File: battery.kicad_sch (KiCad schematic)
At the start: 86 parts, among them J6 Conn_01x02, Q3 AON7534, Q4 AON7534, Q7 TI CSD18512Q5B, SW3 RESET, U10 MAX17320G22+, U9 BQ25798

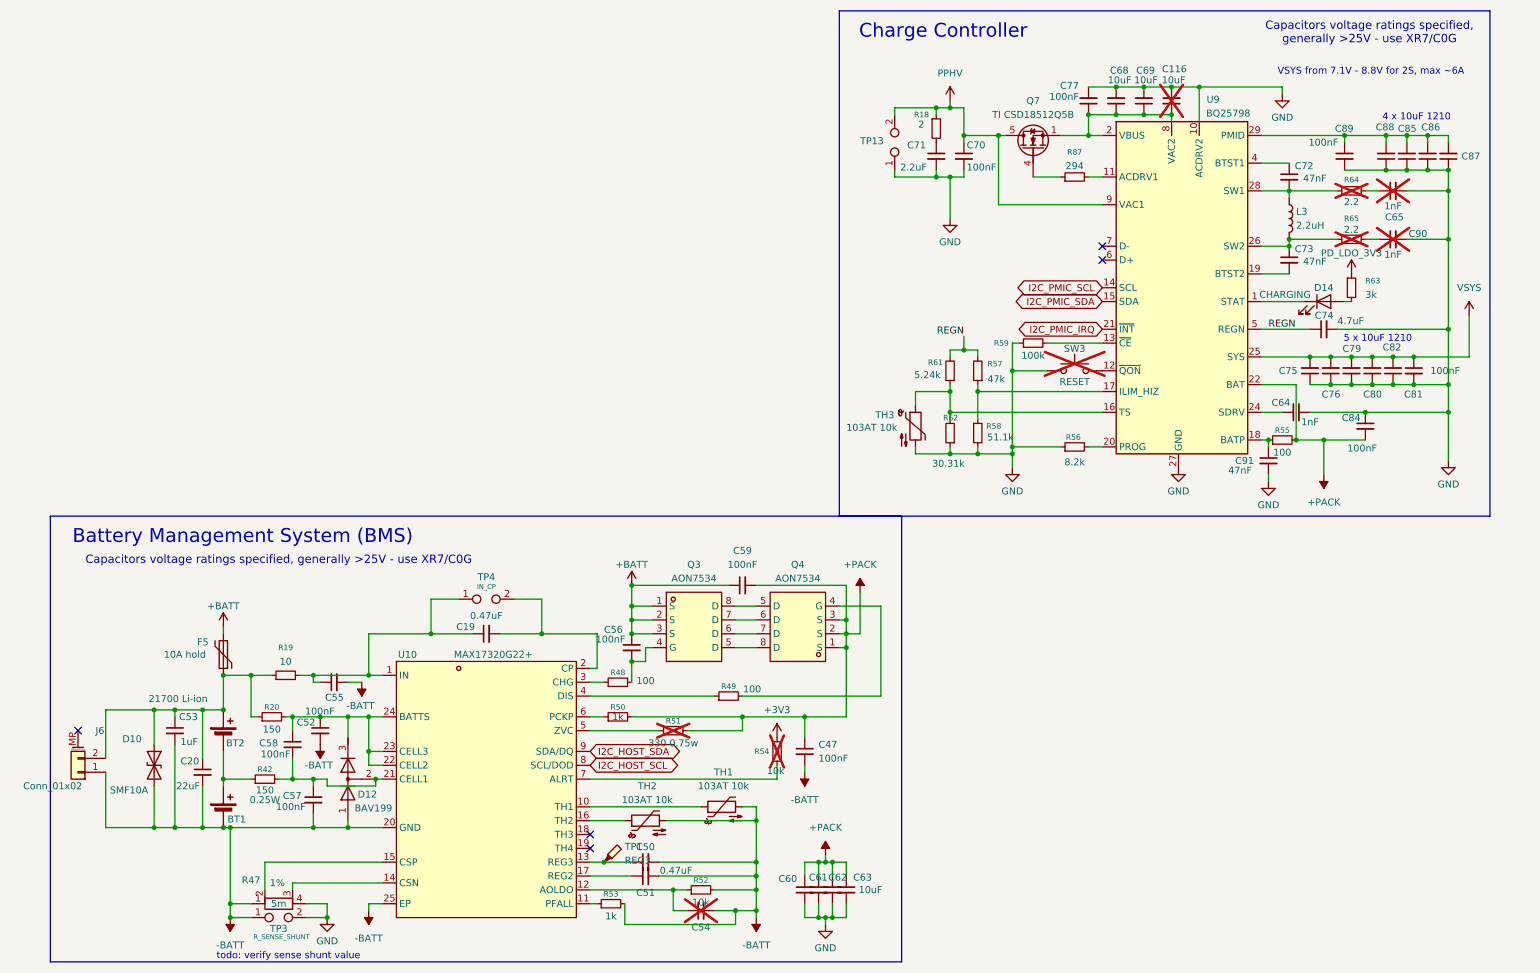
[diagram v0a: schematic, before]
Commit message: push for review, minor changes
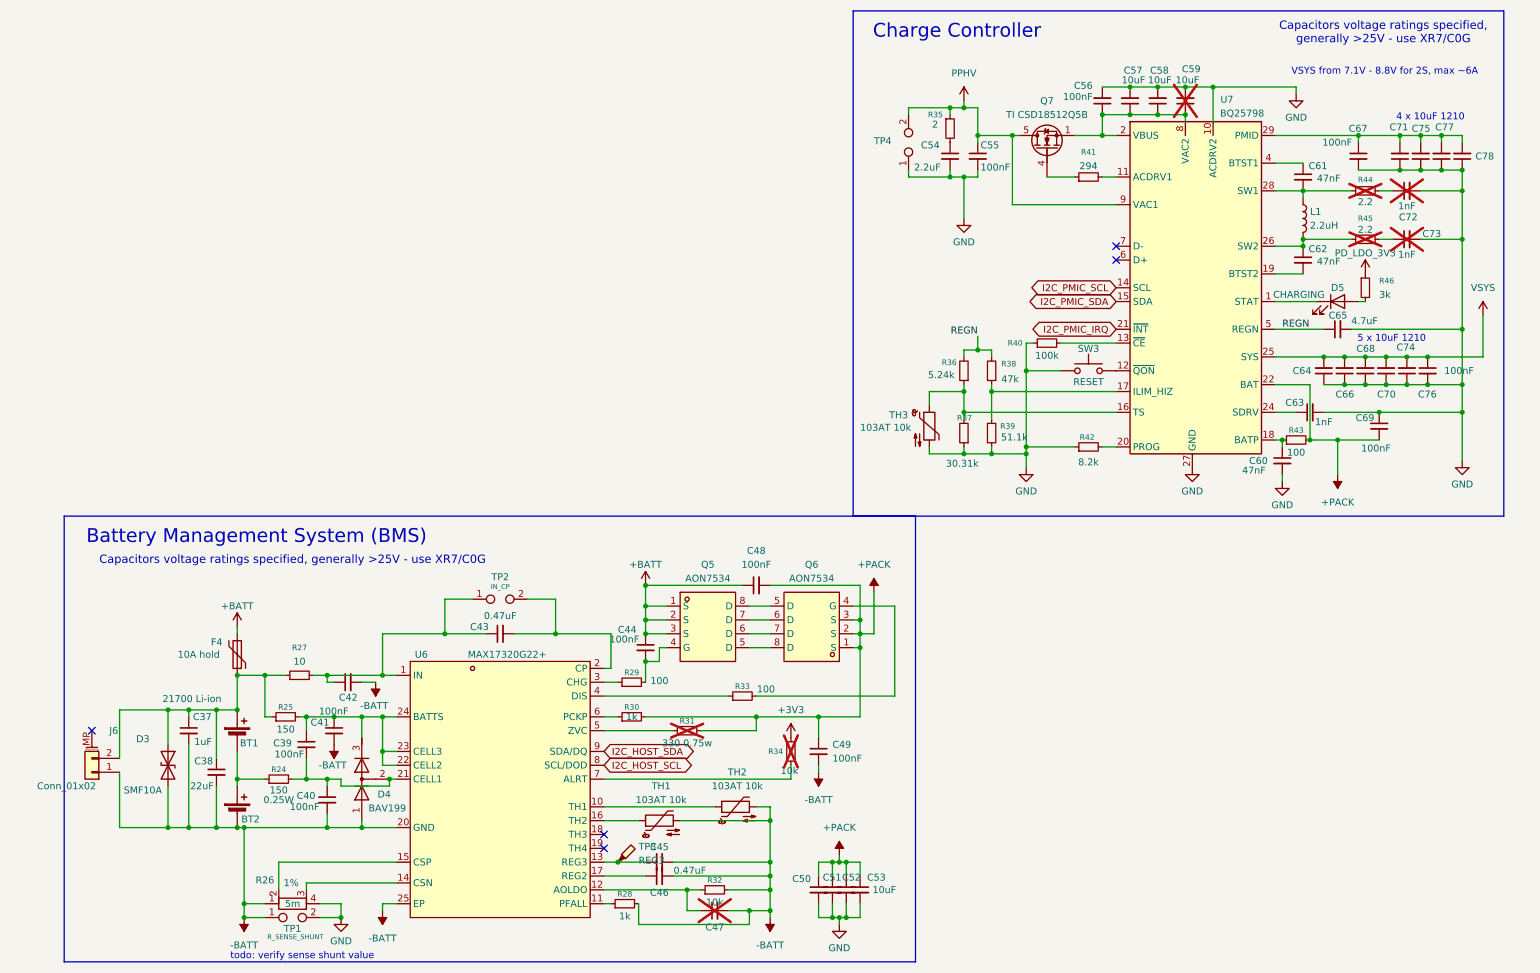
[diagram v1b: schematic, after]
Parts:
- removed C116, C79, C80, C82, C85, C86, C87, C88: 10uF, Capacitor_SMD:C_1210_3225Metric, symbol Device:C_Small
- removed C19: 0.47uF, symbol Device:C_Small
- removed C20: 22uF, Capacitor_SMD:C_0805_2012Metric, symbol Device:C_Small
- removed C81, C84, C89: 100nF, Capacitor_SMD:C_0402_1005Metric, symbol Device:C_Small
- removed C90: 1nF, Capacitor_SMD:C_0402_1005Metric_Pad0.74x0.62mm_HandSolder, symbol Device:C_Small
- removed C91: 47nF, Capacitor_SMD:C_0402_1005Metric, symbol Device:C_Small
- removed D10: SMF10A, Diode_SMD:D_SOD-123, symbol Device:D_TVS
- removed D12: BAV199, Package_TO_SOT_SMD:SOT-23, symbol Device:D_Dual_Series_ACK
- removed D14: CHARGING, symbol Device:LED
- removed F5: 10A hold, symbol Device:Polyfuse
- removed L3: 2.2uH, symbol Device:L
- removed Q3, Q4: AON7534, easyeda2kicad:PQFN-8_L3.1-W3.1-P0.65-LS3.3-BL, symbol easyeda2kicad:AON7534-ES
- removed R18: 2, Resistor_SMD:R_0402_1005Metric, symbol Device:R_Small
- removed R19: 10, symbol Device:R_Small
- removed R20: 150, Resistor_SMD:R_1206_3216Metric, symbol Device:R_Small
- removed R47: 5m, symbol Device:R_Shunt
- removed R48, R49: 100, symbol Device:R_Small
- removed R50, R53: 1k, symbol Device:R_Small
- removed R51: 330 0.75w, Resistor_SMD:R_2010_5025Metric, symbol Device:R_Small
- removed R52, R54: 10k, symbol Device:R_Small
- removed R55: 100, Resistor_SMD:R_0402_1005Metric, symbol Device:R_Small
- removed R56: 8.2k, Resistor_SMD:R_0402_1005Metric_Pad0.72x0.64mm_HandSolder, symbol Device:R_Small
- removed R57: 47k, Resistor_SMD:R_0603_1608Metric_Pad0.98x0.95mm_HandSolder, symbol Device:R_Small
- removed R58: 51.1k, Resistor_SMD:R_0603_1608Metric_Pad0.98x0.95mm_HandSolder, symbol Device:R_Small
- removed R59: 100k, Resistor_SMD:R_0402_1005Metric, symbol Device:R_Small
- removed R61: 5.24k, Resistor_SMD:R_0603_1608Metric_Pad0.98x0.95mm_HandSolder, symbol Device:R_Small
- removed R62: 30.31k, Resistor_SMD:R_0603_1608Metric_Pad0.98x0.95mm_HandSolder, symbol Device:R_Small
- removed R63: 3k, Resistor_SMD:R_0402_1005Metric_Pad0.72x0.64mm_HandSolder, symbol Device:R_Small
- removed R64, R65: 2.2, Resistor_SMD:R_0402_1005Metric_Pad0.72x0.64mm_HandSolder, symbol Device:R_Small
- removed R87: 294, symbol Device:R_Small
- removed TP1: REG3, symbol Connector:TestPoint_Probe
- removed TP13: PPHV, symbol Connector:TestPoint_2Pole
- removed TP3: R_SENSE_SHUNT, TestPoint:TestPoint_2Pads_Pitch2.54mm_Drill0.8mm, symbol Connector:TestPoint_2Pole
- removed U10: MAX17320G22+, easyeda2kicad:QFN-24_L4.0-W4.0-P0.50-BL-EP2.6, symbol easyeda2kicad:MAX17320G22+
- removed U9: BQ25798, Package_DFN_QFN:Texas_RQM0029A_VQFN-29_4x4mm_P0.4mm, symbol Battery_Management:BQ25798
- added C37, C42: 1uF, symbol Device:C_Small
- added C38: 22uF, Capacitor_SMD:C_0805_2012Metric, symbol Device:C_Small
- added C39, C40, C41, C44, C48, C49: 100nF, symbol Device:C_Small
- added C43: 0.47uF, symbol Device:C_Small
- added C45, C46: 0.47uF, Capacitor_SMD:C_0402_1005Metric, symbol Device:C_Small
- added C66, C78: 10uF, Capacitor_SMD:C_1210_3225Metric, symbol Device:C_Small
- added C67: 100nF, Capacitor_SMD:C_0402_1005Metric, symbol Device:C_Small
- added D3: SMF10A, Diode_SMD:D_SOD-123, symbol Device:D_TVS
- added D4: BAV199, Package_TO_SOT_SMD:SOT-23, symbol Device:D_Dual_Series_ACK
- added D5: CHARGING, symbol Device:LED
- added F4: 10A hold, symbol Device:Polyfuse
- added L1: 2.2uH, Inductor_SMD:L_Vishay_IFSC-1515AH_4x4x1.8mm, symbol Device:L
- added Q5, Q6: AON7534, easyeda2kicad:PQFN-8_L3.1-W3.1-P0.65-LS3.3-BL, symbol easyeda2kicad:AON7534-ES
- added R24, R25: 150, Resistor_SMD:R_1206_3216Metric, symbol Device:R_Small
- added R26: 5m, symbol Device:R_Shunt
- added R27: 10, symbol Device:R_Small
- added R28, R30: 1k, symbol Device:R_Small
- added R29, R33: 100, symbol Device:R_Small
- added R31: 330 0.75w, Resistor_SMD:R_2010_5025Metric, symbol Device:R_Small
- added R32, R34: 10k, symbol Device:R_Small
- added R35: 2, Resistor_SMD:R_0402_1005Metric, symbol Device:R_Small
- added R36: 5.24k, Resistor_SMD:R_0603_1608Metric_Pad0.98x0.95mm_HandSolder, symbol Device:R_Small
- added R37: 30.31k, Resistor_SMD:R_0603_1608Metric_Pad0.98x0.95mm_HandSolder, symbol Device:R_Small
- added R38: 47k, Resistor_SMD:R_0603_1608Metric_Pad0.98x0.95mm_HandSolder, symbol Device:R_Small
- added R39: 51.1k, Resistor_SMD:R_0603_1608Metric_Pad0.98x0.95mm_HandSolder, symbol Device:R_Small
- added R40: 100k, Resistor_SMD:R_0402_1005Metric, symbol Device:R_Small
- added R41: 294, symbol Device:R_Small
- added R43: 100, Resistor_SMD:R_0402_1005Metric, symbol Device:R_Small
- added R44, R45: 2.2, Resistor_SMD:R_0402_1005Metric_Pad0.72x0.64mm_HandSolder, symbol Device:R_Small
- added R46: 3k, Resistor_SMD:R_0402_1005Metric_Pad0.72x0.64mm_HandSolder, symbol Device:R_Small
- added TP1: R_SENSE_SHUNT, TestPoint:TestPoint_2Pads_Pitch2.54mm_Drill0.8mm, symbol Connector:TestPoint_2Pole
- added TP2: IN_CP, TestPoint:TestPoint_2Pads_Pitch2.54mm_Drill0.8mm, symbol Connector:TestPoint_2Pole
- added TP3: REG3, symbol Connector:TestPoint_Probe
- added U6: MAX17320G22+, easyeda2kicad:QFN-24_L4.0-W4.0-P0.50-BL-EP2.6, symbol easyeda2kicad:MAX17320G22+
- added U7: BQ25798, Package_DFN_QFN:Texas_RQM0029A_VQFN-29_4x4mm_P0.4mm, symbol Battery_Management:BQ25798
- C47: value 100nF -> 0.47uF; footprint (none) -> Capacitor_SMD:C_0402_1005Metric; Voltage Rating 50V -> 16V; now not fitted
- C50: value 0.47uF -> 10uF; footprint Capacitor_SMD:C_0402_1005Metric -> Capacitor_SMD:C_0805_2012Metric; LCSC Part (none) -> C33546010
- C51: value 0.47uF -> 10uF; footprint Capacitor_SMD:C_0402_1005Metric -> Capacitor_SMD:C_0805_2012Metric; LCSC Part (none) -> C33546010; Voltage Rating 16V -> 25V
- C52: value 100nF -> 10uF; footprint (none) -> Capacitor_SMD:C_0805_2012Metric; LCSC Part (none) -> C33546010; Voltage Rating 50V -> 25V
- C53: value 1uF -> 10uF; footprint (none) -> Capacitor_SMD:C_0805_2012Metric; LCSC Part (none) -> C33546010; Voltage Rating 50V -> 25V
- C54: value 0.47uF -> 2.2uF; footprint Capacitor_SMD:C_0402_1005Metric -> Capacitor_SMD:C_0805_2012Metric; Voltage Rating 16V -> 50V; now fitted
- C55: value 1uF -> 100nF; footprint (none) -> Capacitor_SMD:C_0402_1005Metric; LCSC Part (none) -> C6119785
- C56: footprint (none) -> Capacitor_SMD:C_0402_1005Metric; LCSC Part (none) -> C6119785; Voltage Rating 25V -> 50V
- C57: value 100nF -> 10uF; footprint (none) -> Capacitor_SMD:C_1210_3225Metric; LCSC Part (none) -> C33546018; Voltage Rating 25V -> 50V
- C58: value 100nF -> 10uF; footprint (none) -> Capacitor_SMD:C_1210_3225Metric; LCSC Part (none) -> C33546018
- C59: value 100nF -> 10uF; footprint (none) -> Capacitor_SMD:C_1210_3225Metric; LCSC Part (none) -> C33546018; now not fitted
- C60, C61, C62: value 10uF -> 47nF; footprint Capacitor_SMD:C_0805_2012Metric -> Capacitor_SMD:C_0402_1005Metric; LCSC Part C33546010 -> (none); Voltage Rating 25V -> 50V
- C63: value 10uF -> 1nF; footprint Capacitor_SMD:C_0805_2012Metric -> Capacitor_SMD:C_0402_1005Metric; LCSC Part C33546010 -> (none); Voltage Rating 25V -> 50V
- C64: value 1nF -> 10uF; footprint Capacitor_SMD:C_0402_1005Metric -> Capacitor_SMD:C_1210_3225Metric; LCSC Part (none) -> C7472976
- C65: value 1nF -> 4.7uF; footprint Capacitor_SMD:C_0402_1005Metric_Pad0.74x0.62mm_HandSolder -> Capacitor_SMD:C_0603_1608Metric; Voltage Rating 50V -> 16V; now fitted; now in the parts list
- C68: LCSC Part C33546018 -> C7472976
- C69: value 10uF -> 100nF; footprint Capacitor_SMD:C_1210_3225Metric -> Capacitor_SMD:C_0402_1005Metric; LCSC Part C33546018 -> C6119785
- C70, C77: value 100nF -> 10uF; footprint Capacitor_SMD:C_0402_1005Metric -> Capacitor_SMD:C_1210_3225Metric; LCSC Part C6119785 -> C7472976
- C71: value 2.2uF -> 10uF; footprint Capacitor_SMD:C_0805_2012Metric -> Capacitor_SMD:C_1210_3225Metric; LCSC Part (none) -> C7472976
- C72, C73: value 47nF -> 1nF; footprint Capacitor_SMD:C_0402_1005Metric -> Capacitor_SMD:C_0402_1005Metric_Pad0.74x0.62mm_HandSolder; now not fitted; now left out of the parts list
- C74: value 4.7uF -> 10uF; footprint Capacitor_SMD:C_0603_1608Metric -> Capacitor_SMD:C_1210_3225Metric; LCSC Part (none) -> C7472976; Voltage Rating 16V -> 50V
- C76: value 10uF -> 100nF; footprint Capacitor_SMD:C_1210_3225Metric -> Capacitor_SMD:C_0402_1005Metric; LCSC Part C7472976 -> C6119785
- R42: value 150 -> 8.2k; footprint Resistor_SMD:R_1206_3216Metric -> Resistor_SMD:R_0402_1005Metric_Pad0.72x0.64mm_HandSolder; Power Rating 0.25W -> (none); Tolerance (none) -> 1%
- SW3: now fitted
- TP4: value IN_CP -> PPHV; footprint TestPoint:TestPoint_2Pads_Pitch2.54mm_Drill0.8mm -> (none)
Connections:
- net +3V3: now also R34.2
- net +BATT: now also C44.1, C48.1, F4.2, Q5.1 (S), Q5.2 (S), Q5.3 (S); no longer C56.1, C59.1
- net +PACK: now also C50.1, C51.1, C52.1, C53.1, C69.2, C48.2, C49.1, Q6.1 (S), Q6.2 (S), Q6.3 (S), R30.2, R31.2, R43.2, U7.22 (BAT), U7.23 (BAT); no longer C47.1, C59.2, C60.1, C61.1, C62.1, C63.1
- net -BATT: now also BT2.2 (-), C37.2, C38.2, C40.2, C41.2, C42.2, C45.2, C46.2, C49.2, D3.2 (A2), D4.1 (A), R26.1, R28.2, R32.2, TP1.1, U6.20 (GND), U6.25 (EP); no longer BT1.2 (-), C50.2, C51.2, C52.2, C53.2, C54.2, C55.2, C57.2
- net GND: now also C50.2, C51.2, C52.2, C53.2, C54.2, C55.2, C56.2, C57.2, C58.2, C59.2, C64.1, C68.1, C69.1, C70.1, C71.1, C72.2, C73.2, C74.1, C76.2, C77.1, R42.1, TP4.1, C66.1, C67.2, C78.1, R26.4, R37.1, R39.2, R40.1, TP1.2, U7.10 (ACDRV2), U7.27 (GND); no longer C61.2, C62.2, C64.2, C68.2, C69.2, C70.2, C71.2, C74.2, C76.1, C77.2
- net I2C_HOST_SCL: now also U6.8 (SCL/DOD)
- net I2C_HOST_SDA: now also U6.9 (SDA/DQ)
- net I2C_PMIC_IRQ: now also U7.21 (~{INT})
- net I2C_PMIC_SCL: now also U7.14 (SCL)
- net I2C_PMIC_SDA: now also U7.15 (SDA)
- net PD_LDO_3V3: now also R46.1
- net PPHV: now also C55.1, TP4.2, R35.1, U7.9 (VAC1); no longer C70.1
- net REGN: now also C65.1, R36.2, R38.2, U7.5 (REGN); no longer C74.1
- net VSYS: now also C64.2, C68.2, C70.2, C74.2, C76.1, C66.2, U7.25 (SYS); no longer C75.2, C76.2
- net at Q7.1 (S), Q7.2 (S), Q7.3 (S): now also C56.1, C57.1, C58.1, C59.1, U7.2 (VBUS), U7.3 (VBUS), U7.8 (VAC2); no longer C68.1, C69.1, C77.1
- net at Q7.4 (G): now also R41.1
- net at TH3.1: now also R36.1, R37.2, U7.16 (TS)
- net at TH1.1: now also U6.16 (TH2)
- net at SW3.2: now also U7.12 (~{QON})
- net at C72.1: now also R44.2
- net at C54.1: now also R35.2
- net at C73.1: now also R45.2
- net at TH2.1: now also U6.10 (TH1)
- new net: R26.2, U6.15 (CSP)
- new net: R26.3, U6.14 (CSN)
- new net: C60.1, R43.1, U7.18 (BATP)
- new net: C45.1, TP3.1, U6.13 (REG3)
- new net: BT1.1 (+), C37.1, C38.1, D3.1 (A1), F4.1, J6.2 (Pin_2), R25.1, R27.1
- new net: C62.1, L1.2, R45.1, U7.26 (SW2)
- new net: R40.2, U7.13 (~{CE})
- new net: C39.2, C40.1, D4.2 (common), R24.2, U6.21 (CELL1)
- new net: C39.1, C41.1, D4.3 (K), R25.2, U6.22 (CELL2), U6.23 (CELL3), U6.24 (BATTS)
- new net: R31.1, U6.5 (ZVC)
- new net: BT1.2 (-), BT2.1 (+), R24.1
- new net: C63.1, U7.24 (SDRV)
- new net: C62.2, U7.19 (BTST2)
- new net: C42.1, C43.1, R27.2, TP2.1, U6.1 (IN)
- new net: R28.1, U6.11 (PFALL)
- new net: C47.1, R32.1, U6.12 (AOLDO)
- new net: C46.1, U6.17 (REG2)
- new net: C43.2, TP2.2, U6.2 (CP)
- new net: R29.1, U6.3 (CHG)
- new net: R33.1, U6.4 (DIS)
- new net: R30.1, U6.6 (PCKP)
- new net: R34.1, U6.7 (ALRT)
- new net: C67.1, C71.2, C75.2, C77.2, C78.2, U7.29 (PMID)
- new net: Q6.4 (G), R33.2
- new net: Q5.8 (D), Q6.5 (D)
- new net: Q5.7 (D), Q6.6 (D)
- new net: Q5.6 (D), Q6.7 (D)
- new net: Q5.5 (D), Q6.8 (D)
- new net: R38.1, R39.1, U7.17 (ILIM_HIZ)
- new net: D5.1 (K), U7.1 (STAT)
- new net: R41.2, U7.11 (ACDRV1)
- new net: R42.2, U7.20 (PROG)
- new net: C61.2, L1.1, R44.1, U7.28 (SW1)
- new net: C61.1, U7.4 (BTST1)
- new net: C44.2, Q5.4 (G), R29.2
- new net: D5.2 (A), R46.2
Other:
- title: Battery Charger / Battery Managment System -> Battery Charger / Battery Managment System (BMS)
